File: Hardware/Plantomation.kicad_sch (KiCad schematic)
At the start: 92 parts, among them J1 12V, J10 ADC1_0, J11 Valve 3, J12 Valve 4, J13 Ch_Sel, J14 GSD090012SEU, J2 USB_B, J3 ADC1_4, J4 ADC1_5, J5 ADC1_6, J6 ADC1_7, J7 PeriPump, J8 Valve 1, J9 Valve 2, Q1 BC846, Q2 DMG1012UW7, Q3 BC846, Q4 BSS138, Q5 BSS138, Q6 BSS138, Q7 BSS138, SW1 RST, SW2 BOOT, U1 ESP32-WROOM-32, U2 USBLC6-2SC6, U3 L7805, U4 AMS1117-3.3, U5 CP2102N-Axx-xQFN28

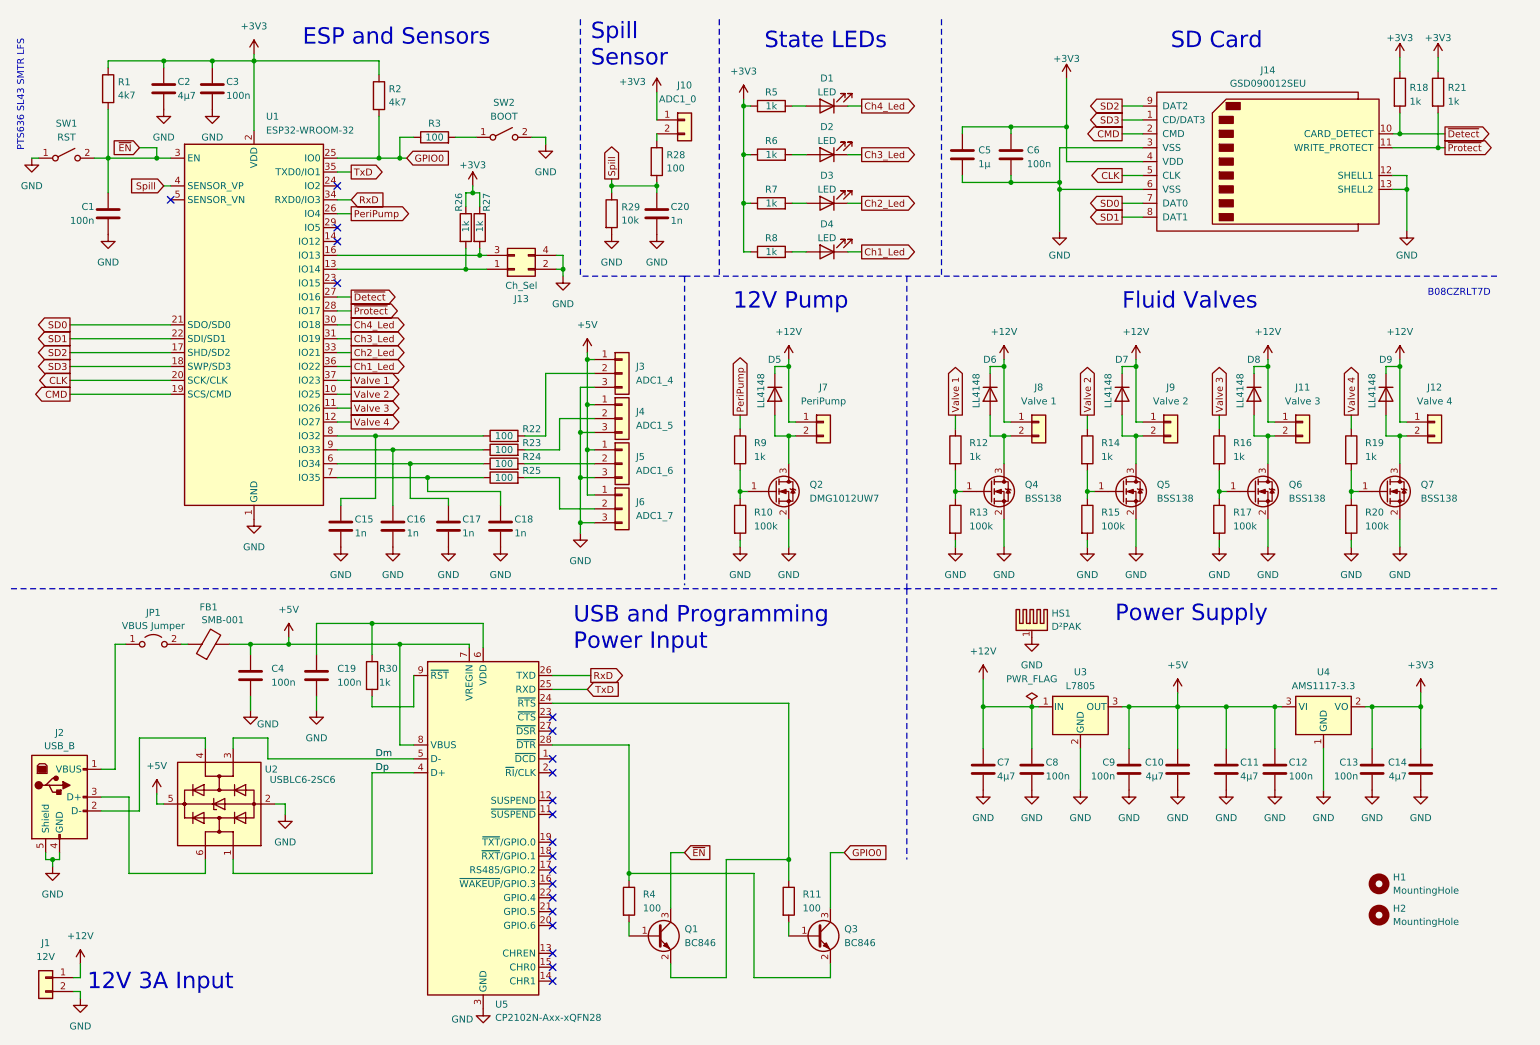
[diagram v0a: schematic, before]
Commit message: codebase and first part review
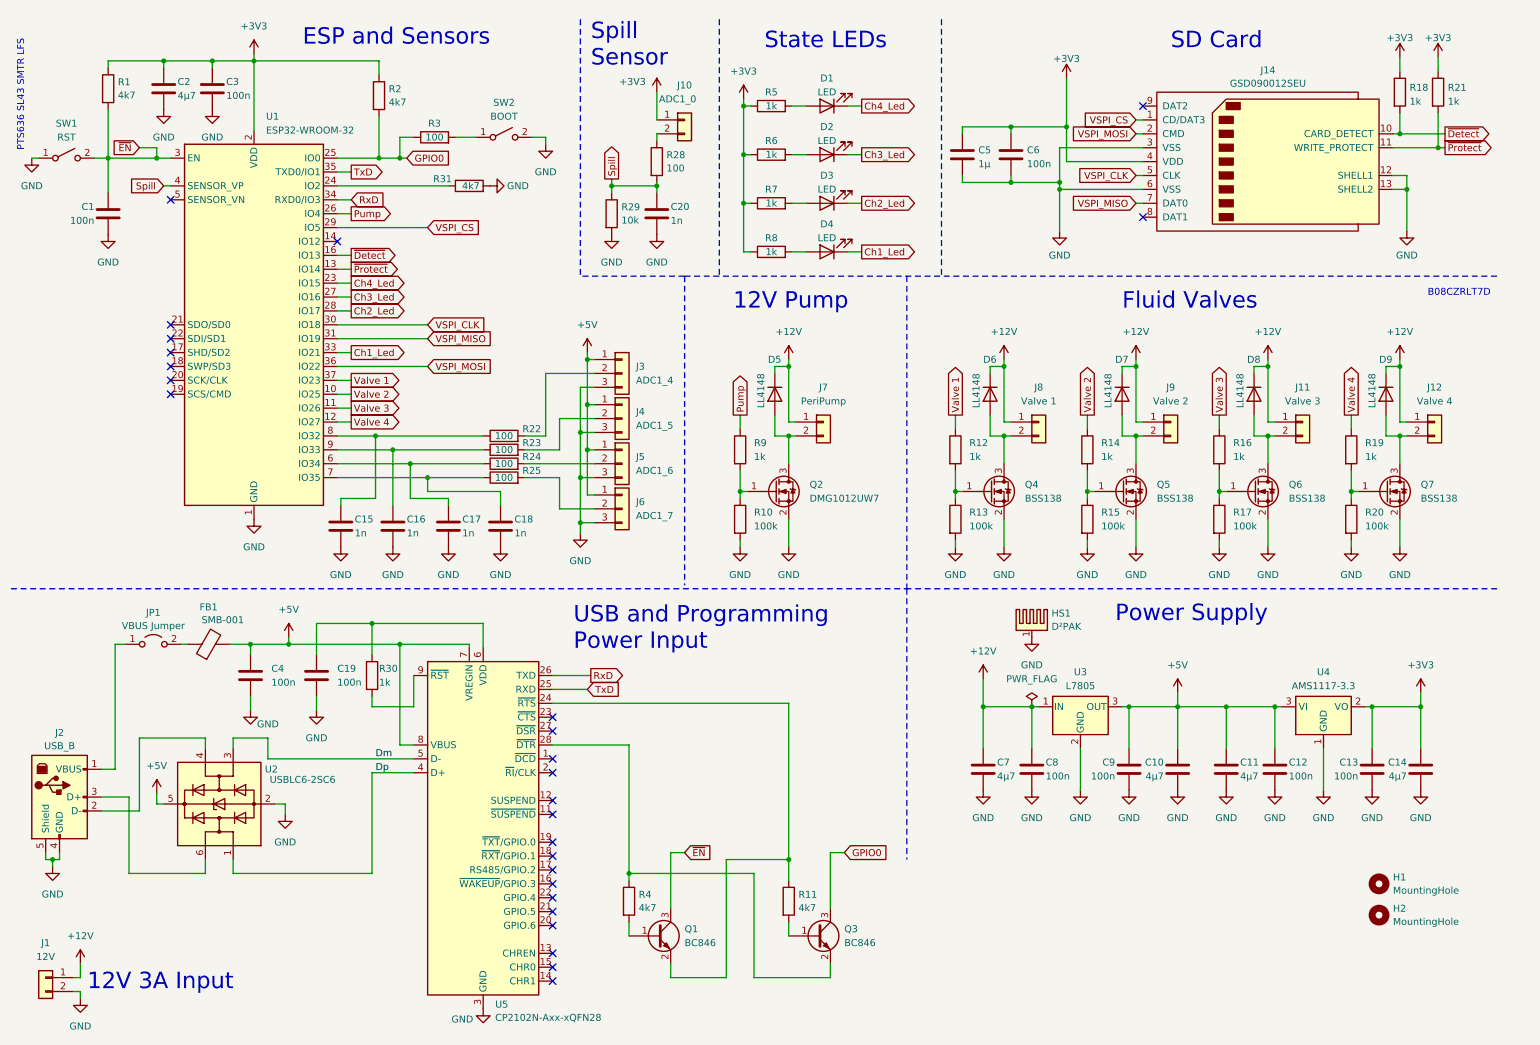
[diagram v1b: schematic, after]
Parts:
- removed J13: Ch_Sel, Connector_PinHeader_2.54mm:PinHeader_2x02_P2.54mm_Vertical, symbol Connector_Generic:Conn_02x02_Odd_Even
- removed R26, R27: 1k, Resistor_SMD:R_0805_2012Metric, symbol Device:R
- added R31: 4k7, Resistor_SMD:R_0805_2012Metric, symbol Device:R
- R11, R4: value 100 -> 4k7
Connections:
- net Ch1_Led: now also U1.33 (IO21); no longer U1.36 (IO22)
- net Ch2_Led: now also U1.28 (IO17); no longer U1.33 (IO21)
- net Ch3_Led: now also U1.27 (IO16); no longer U1.31 (IO19)
- net Ch4_Led: now also U1.23 (IO15); no longer U1.30 (IO18)
- net GND: now also R31.2
- net ~{Detect}: now also U1.16 (IO13); no longer U1.27 (IO16)
- net ~{Protect}: now also U1.13 (IO14); no longer U1.28 (IO17)
- net at U1.24 (IO2): now also R31.1
- net VSPI_CS: now reaches U1.29 (IO5)
- net VSPI_CS: now also J14.1 (CD/DAT3)
- net CLK: no longer names the net of U1.20 (SCK/CLK)
- net CLK: no longer J14.5 (CLK)
- net CMD: no longer names the net of U1.19 (SCS/CMD)
- net CMD: no longer J14.2 (CMD)
- net PeriPump renamed Pump
- net SD0: no longer names the net of U1.21 (SDO/SD0)
- net SD0: no longer J14.7 (DAT0)
- net SD1: no longer names the net of J14.8 (DAT1)
- net SD1: no longer U1.22 (SDI/SD1)
- net SD2: no longer names the net of J14.9 (DAT2)
- net SD2: no longer U1.17 (SHD/SD2)
- net SD3: no longer names the net of U1.18 (SWP/SD3)
- net SD3: no longer J14.1 (CD/DAT3)
- new net VSPI_CLK: J14.5 (CLK), U1.30 (IO18)
- new net VSPI_MISO: J14.7 (DAT0), U1.31 (IO19)
- new net VSPI_MOSI: J14.2 (CMD), U1.36 (IO22)
- no-connect marks 21 -> 26
